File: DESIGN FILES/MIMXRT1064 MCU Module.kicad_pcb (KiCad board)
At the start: 2 copper layers, 40.1 x 40 mm, 106 parts, among them J1 TF-15x15, Q1 IRLML6401, U1 MIMXRT1064CVL5B, U2 IS42S16160J-6BLI, U3 IS25WP064A-JBLE, U4 WM8978CGEFL/RV, U5 UM805RE, U6 UM803RS, Y1 24MHz, Y2 32.768KHz

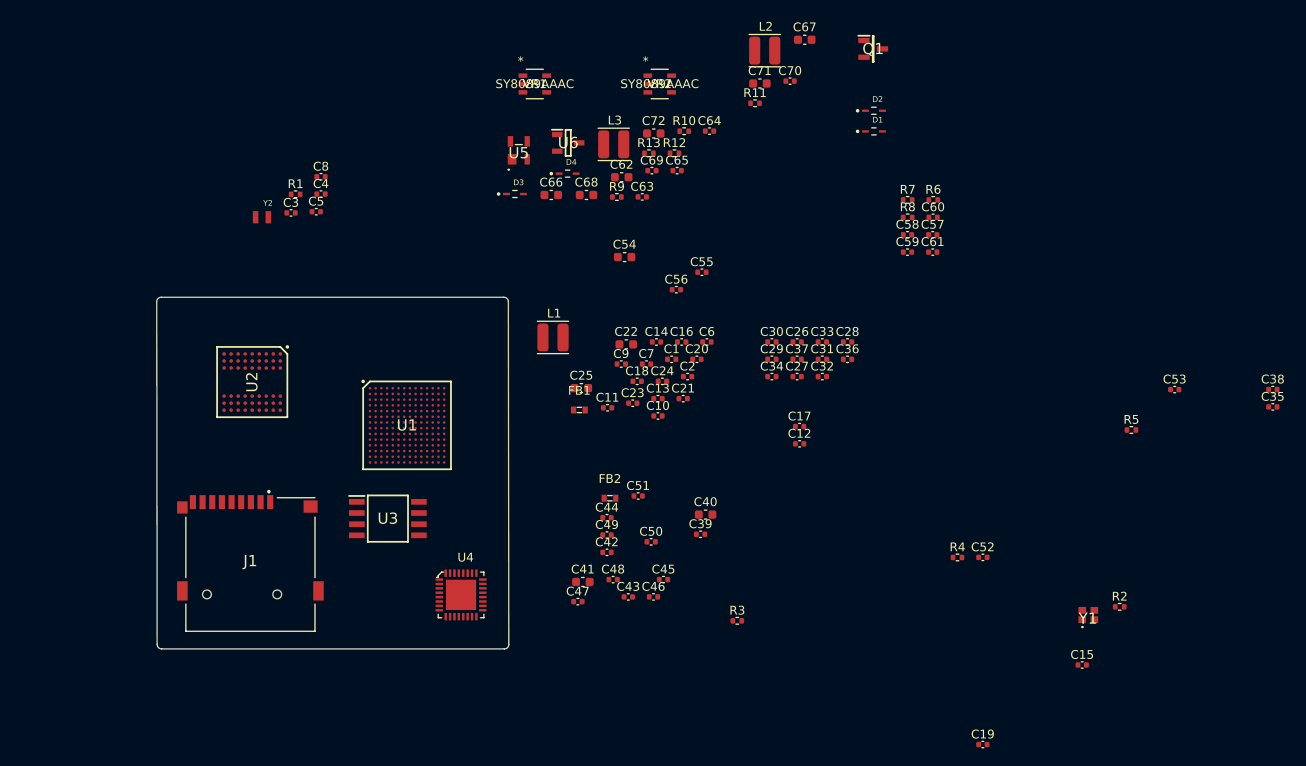
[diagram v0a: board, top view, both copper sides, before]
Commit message: edits
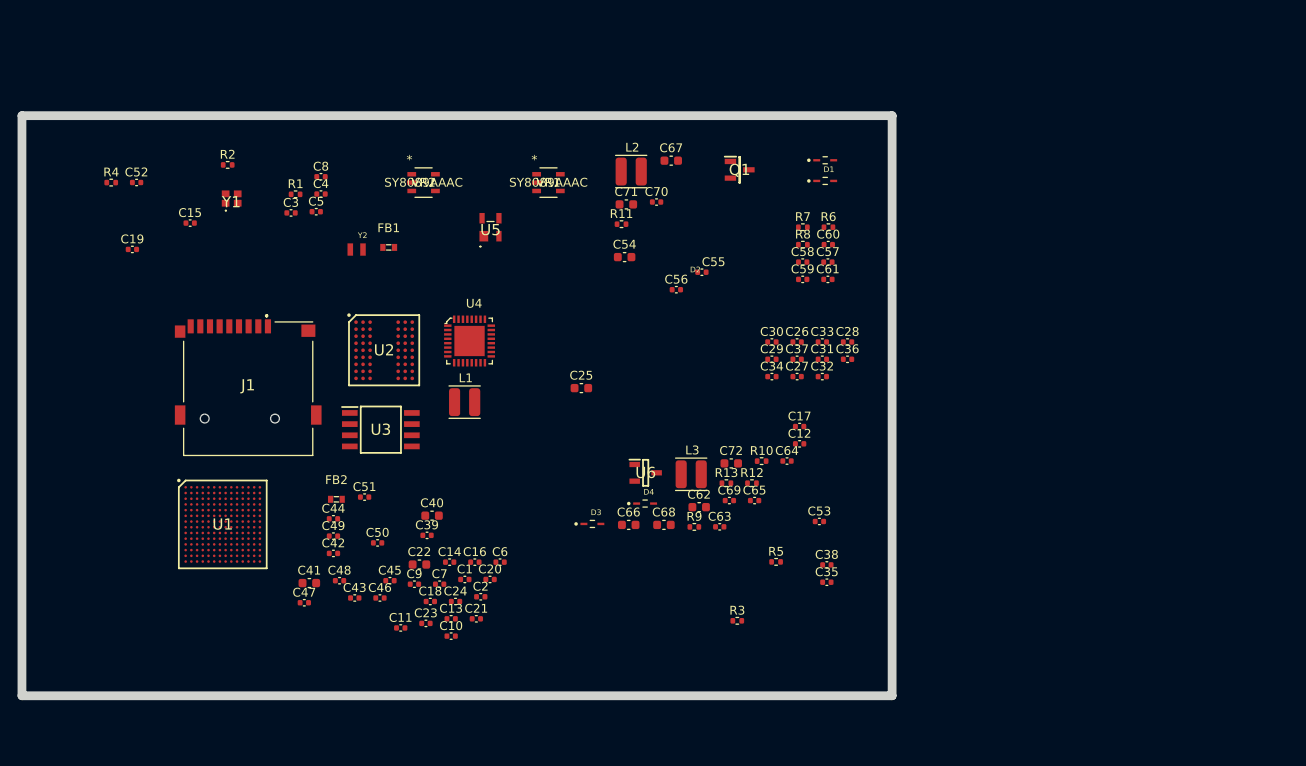
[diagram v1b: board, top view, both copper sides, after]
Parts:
- FB1: value 120R -> BLM18AG121SN1D
- Y1: value 24MHz -> XL7EL89CMI-111YLC-24M
- Y2: value 32.768KHz -> X201232768KJD2SI
- moved C15 113.3 mm to (151.2, 63.0)
- moved R2 113.3 mm to (155.5, 56.4)
- moved C19 112.0 mm to (144.7, 66.0)
- moved Y1 108.4 mm to (156.0, 60.2)
- moved C52 105.4 mm to (145.1, 58.4)
- moved R4 105.4 mm to (142.2, 58.4)
- moved C35 54.6 mm to (223.7, 103.9)
- moved C38 54.6 mm to (223.7, 101.9)
- moved R5 43.1 mm to (217.9, 101.6)
- moved C53 43.1 mm to (222.9, 97.0)
- moved D4 38.6 mm to (203.0, 95.0)
- moved L3 38.6 mm to (208.3, 93.2)
- moved R10 38.6 mm to (216.3, 90.1)
- moved U6 38.6 mm to (203.1, 91.5)
- moved C62 38.6 mm to (209.2, 95.4)
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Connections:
- Y1 pad 2: (no net) -> GND
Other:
- board size 40.1 x 40 mm -> 99.1 x 66 mm
